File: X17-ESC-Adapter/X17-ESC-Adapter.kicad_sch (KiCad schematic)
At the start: 9 parts, among them J2 Power In/Out

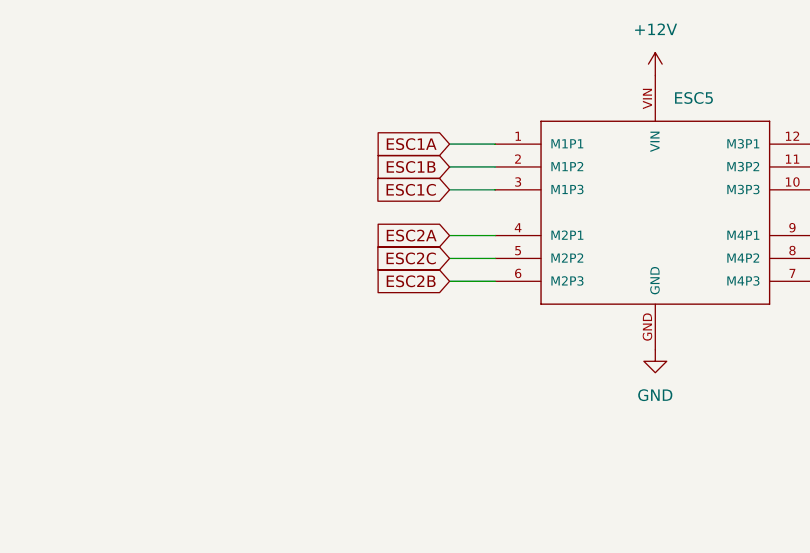
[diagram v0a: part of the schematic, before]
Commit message: 10/12/24
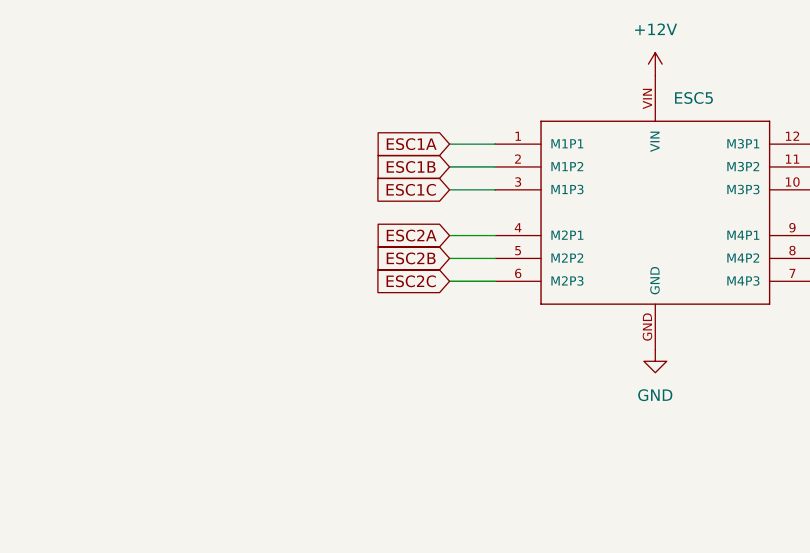
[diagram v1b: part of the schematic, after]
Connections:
- net ESC2B: now also ESC5.5 (M2P2); no longer ESC5.6 (M2P3)
- net ESC2C: now also ESC5.6 (M2P3); no longer ESC5.5 (M2P2)

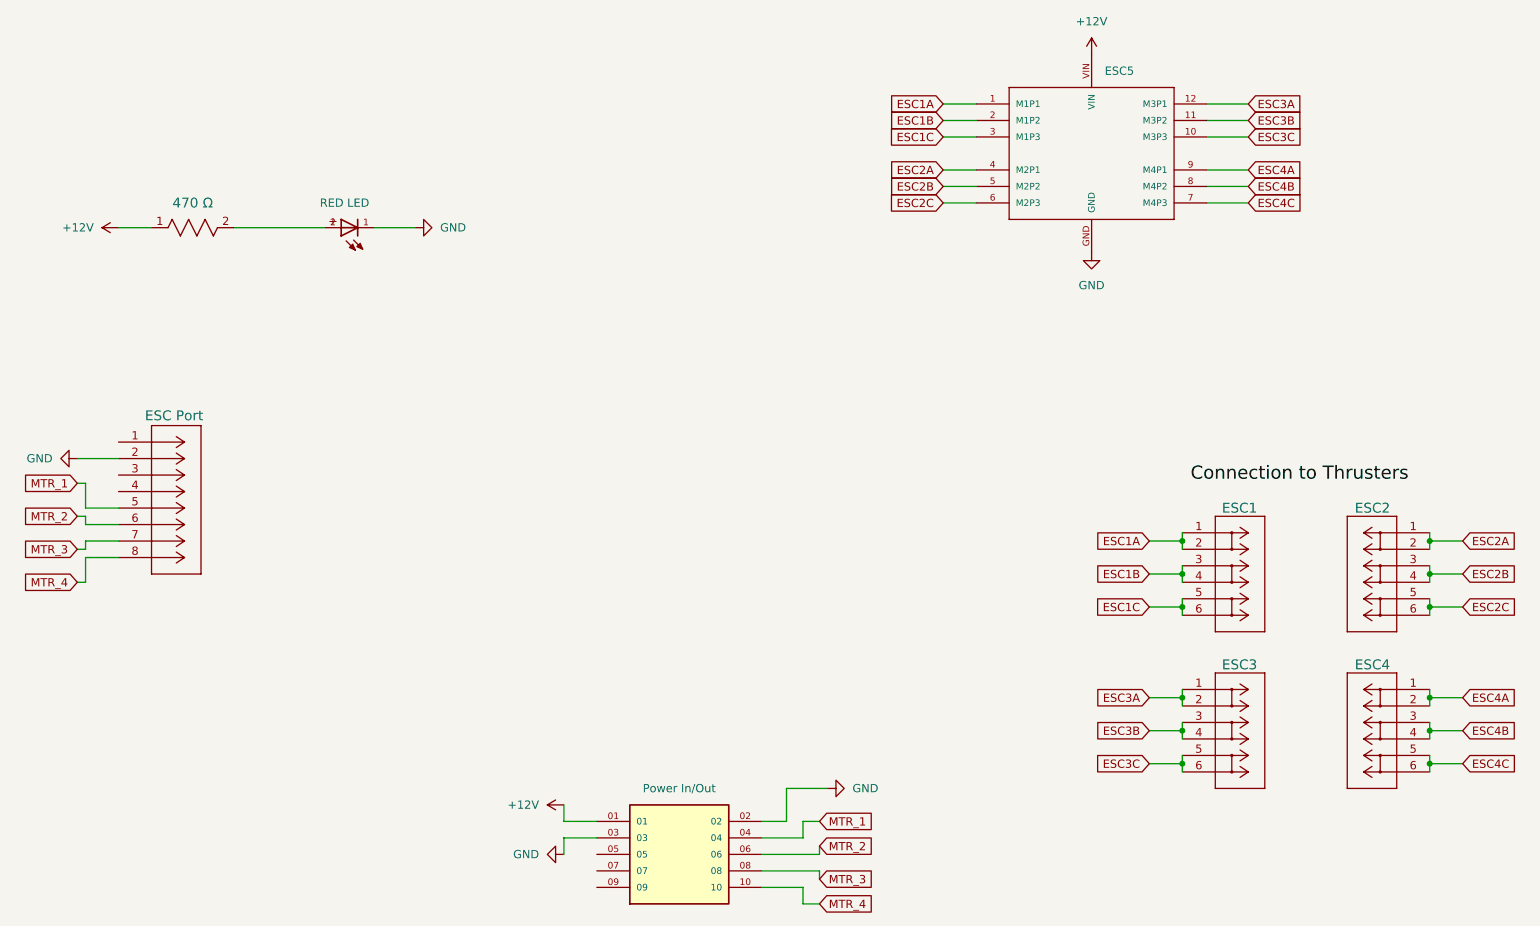
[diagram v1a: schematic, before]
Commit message: before design review
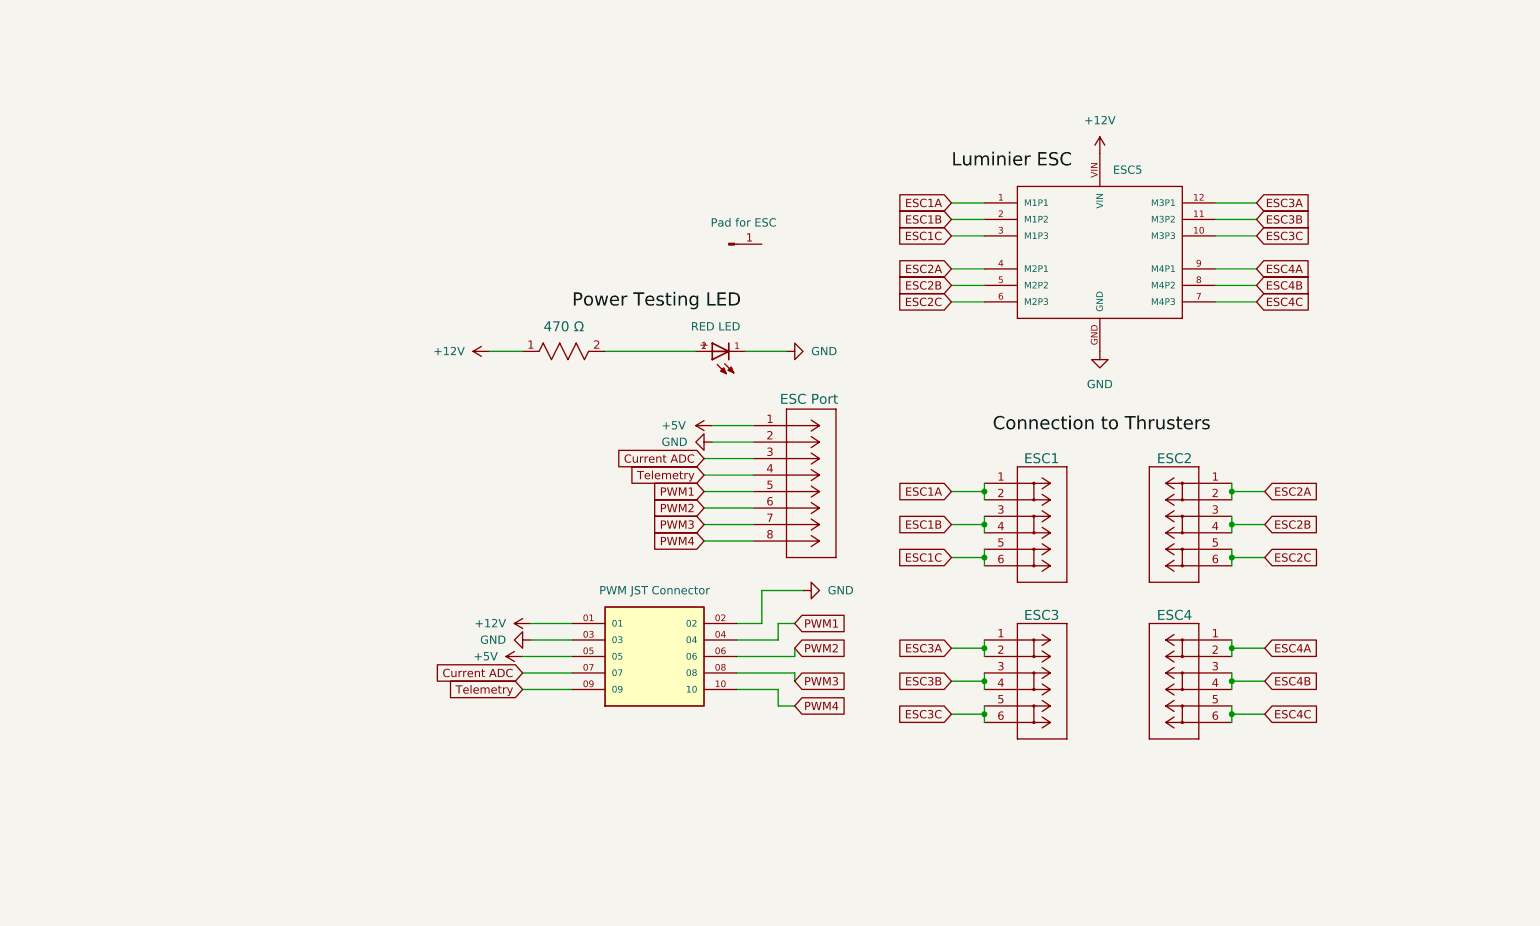
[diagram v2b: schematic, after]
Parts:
- added J1: Pad for ESC, Connector_Wire:SolderWirePad_1x01_SMD_1x2mm, symbol Connector:Conn_01x01_Pin
- J2: value Power In/Out -> PWM JST Connector
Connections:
- net +5V: now reaches BM08B-SRSS-TBLFSN1.1
- net +5V: now also J2.05
- net Current ADC: now reaches BM08B-SRSS-TBLFSN1.3
- net Current ADC: now also J2.07
- net Telemetry: now reaches BM08B-SRSS-TBLFSN1.4
- net Telemetry: now also J2.09
- net MTR_1 renamed PWM1
- net MTR_2 renamed PWM2
- net MTR_3 renamed PWM3
- net MTR_4 renamed PWM4
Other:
- moved on the sheet: ESC1, ESC2, ESC3, ESC4, ESC5

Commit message: made some changes
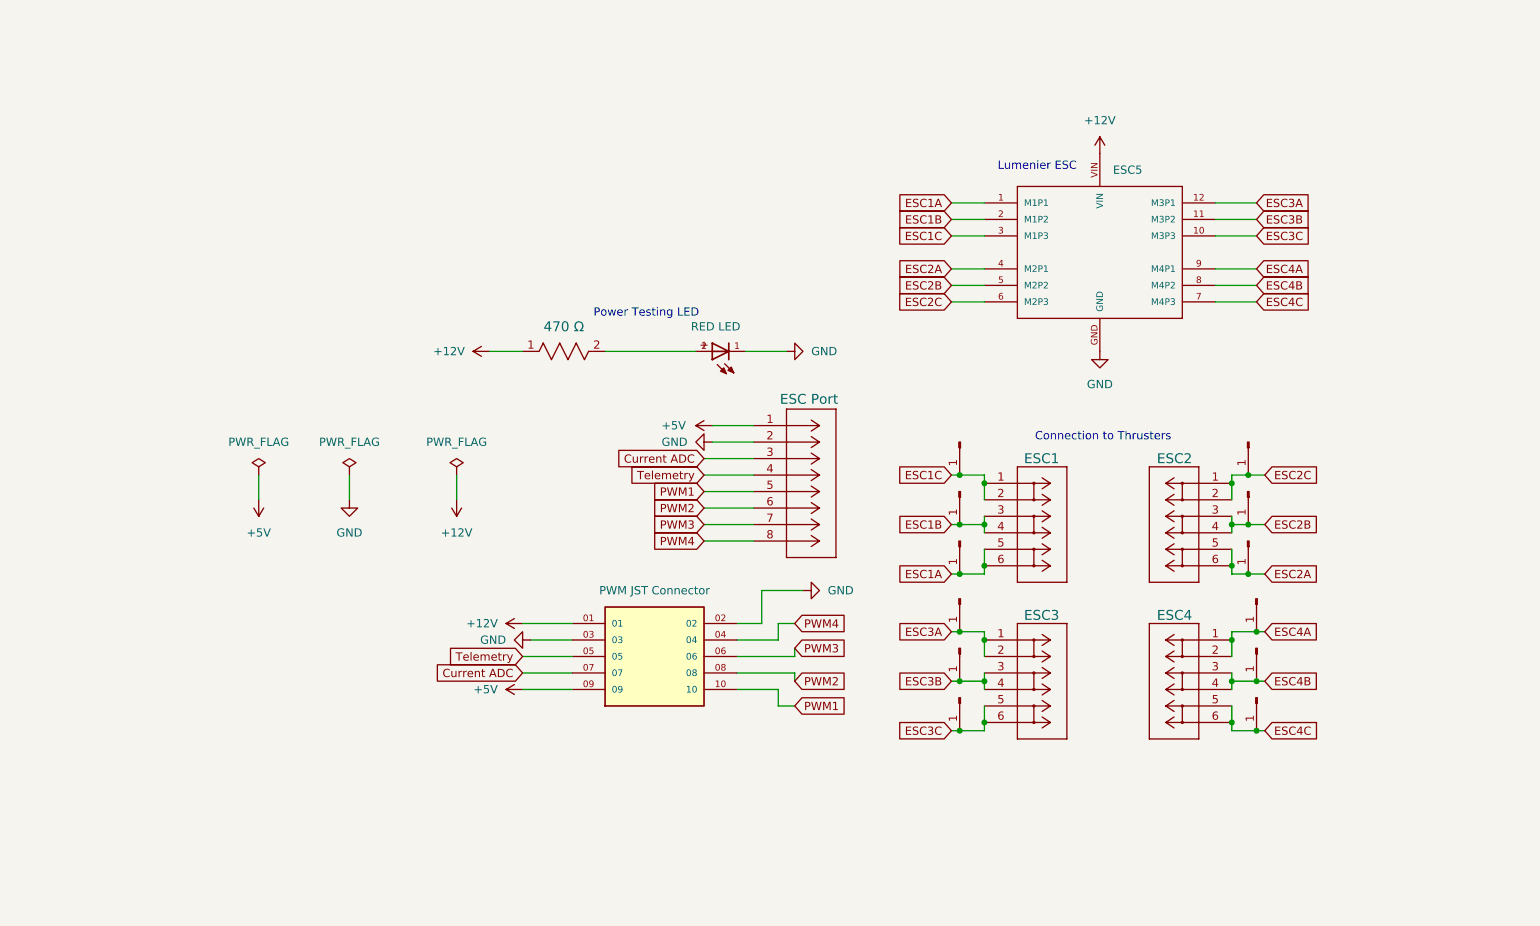
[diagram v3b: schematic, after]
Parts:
- added J10, J11, J12, J13, J3, J4, J5, J6, J7, J8, J9: Pad for ESC, Custom ROV Parts:Pad for ESC Adapter, symbol Connector:Conn_01x01_Pin
- J1: footprint Connector_Wire:SolderWirePad_1x01_SMD_1x2mm -> Custom ROV Parts:Pad for ESC Adapter
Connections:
- net +5V: now also J2.09; no longer J2.05
- net ESC1A: now also ESC1.5, ESC1.6, J4.1 (Pin_1); no longer ESC1.1, ESC1.2
- net ESC1B: now also J3.1 (Pin_1)
- net ESC1C: now also ESC1.1, ESC1.2, J1.1 (Pin_1); no longer ESC1.5, ESC1.6
- net ESC2A: now also ESC2.5, ESC2.6, J7.1 (Pin_1); no longer ESC2.1, ESC2.2
- net ESC2B: now also J6.1 (Pin_1)
- net ESC2C: now also ESC2.1, ESC2.2, J5.1 (Pin_1); no longer ESC2.5, ESC2.6
- net ESC3A: now also J8.1 (Pin_1)
- net ESC3B: now also J10.1 (Pin_1)
- net ESC3C: now also J9.1 (Pin_1)
- net ESC4A: now also J11.1 (Pin_1)
- net ESC4B: now also J12.1 (Pin_1)
- net ESC4C: now also J13.1 (Pin_1)
- net PWM1: now also J2.10; no longer J2.04
- net PWM2: now also J2.08; no longer J2.06
- net PWM3: now also J2.06; no longer J2.08
- net PWM4: now also J2.04; no longer J2.10
- net Telemetry: now also J2.05; no longer J2.09
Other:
- note added: "Connection to Thrusters"
- note added: "Lumenier ESC"
- note added: "Power Testing LED"
